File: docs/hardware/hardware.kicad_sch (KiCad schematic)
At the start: 16 parts, among them J1 BASYS_JA, J2 AudioJack2, J3 GAMEPAD, J6 BASYS_JB, J7 GAMEPAD_1, J8 GAMEPAD_2, SW1 LEFT, SW2 UP, SW3 RIGHT, SW4 PRIMARY, SW5 SECONDARY, SW6 DOWN, SW7 STM_PWR_SOURCE

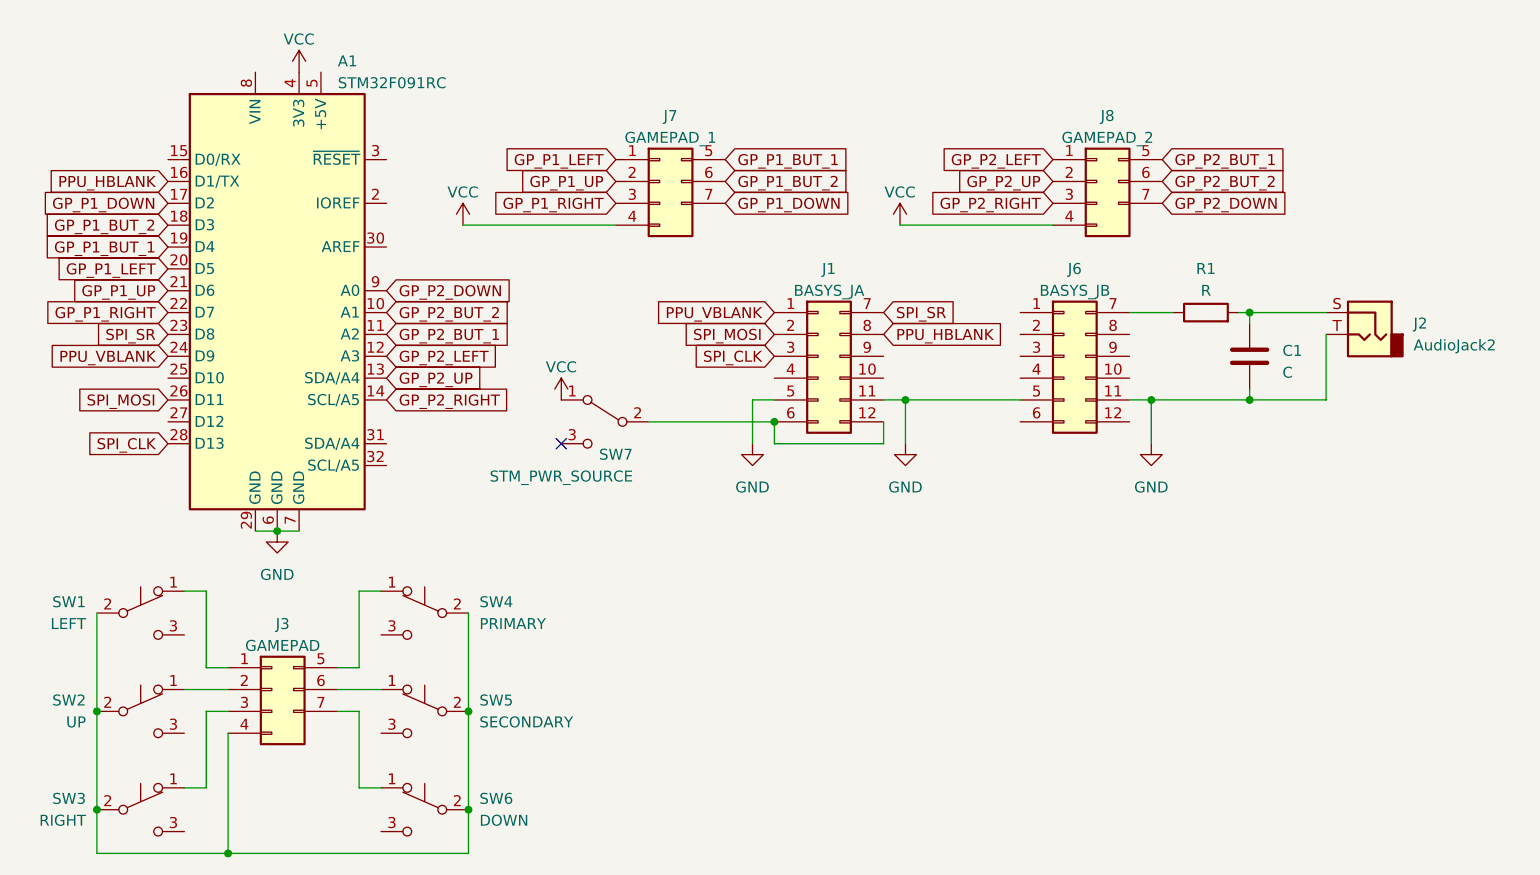
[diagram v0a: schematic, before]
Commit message: final I/O edits
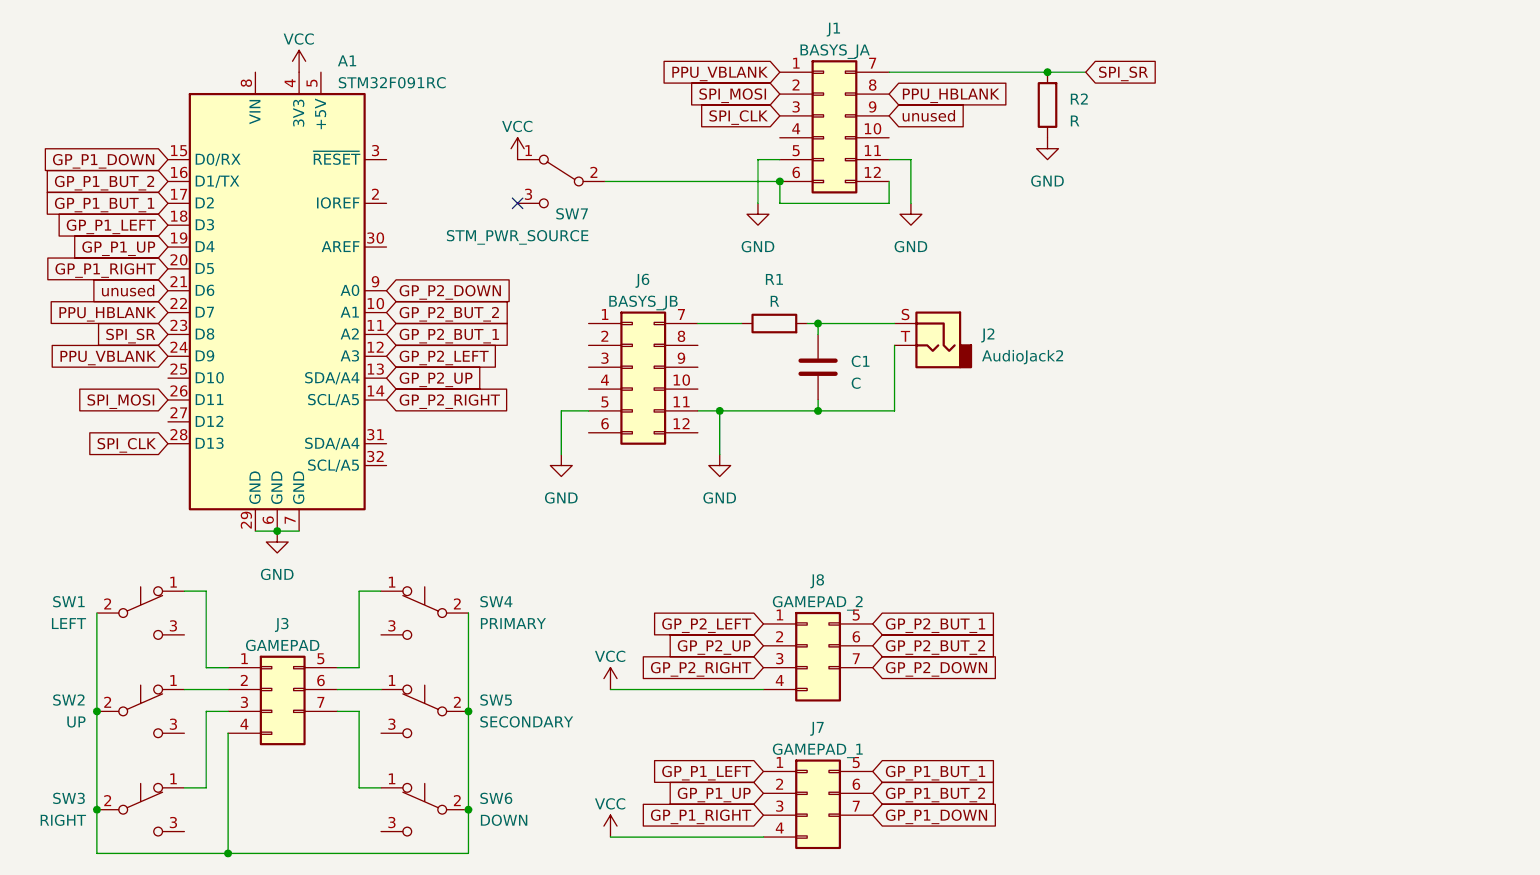
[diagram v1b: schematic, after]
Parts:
- added R2: R, Resistor_THT:R_Axial_DIN0207_L6.3mm_D2.5mm_P7.62mm_Horizontal, symbol Device:R
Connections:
- net GND: now also R2.1
- net GP_P1_BUT_1: now also A1.17 (D2); no longer A1.19 (D4)
- net GP_P1_BUT_2: now also A1.16 (D1/TX); no longer A1.18 (D3)
- net GP_P1_DOWN: now also A1.15 (D0/RX); no longer A1.17 (D2)
- net GP_P1_LEFT: now also A1.18 (D3); no longer A1.20 (D5)
- net GP_P1_RIGHT: now also A1.20 (D5); no longer A1.22 (D7)
- net GP_P1_UP: now also A1.19 (D4); no longer A1.21 (D6)
- net PPU_HBLANK: now also A1.22 (D7); no longer A1.16 (D1/TX)
- net SPI_SR: now also R2.2
- net unused: now reaches J1.9 (Pin_9)
- net unused: now also A1.21 (D6)
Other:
- moved on the sheet: C1, J1, J2, J6, J7, J8, R1, SW7
